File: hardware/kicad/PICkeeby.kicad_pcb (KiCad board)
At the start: 4 copper layers, 85.7 x 55.9 mm, 35 parts, among them J1 PS/2 Connector, J2 PS/2 Connector, J3 MODE_SELECT, J4 Host Interface, J5 Conn_PIC_ICSP_ICD, J6 PS/2 Header, J7 PS/2 Header, U1 PIC16F18344-P, U2 74HCT574, U3 74HCT373, U4 ATF22V10C-10PC

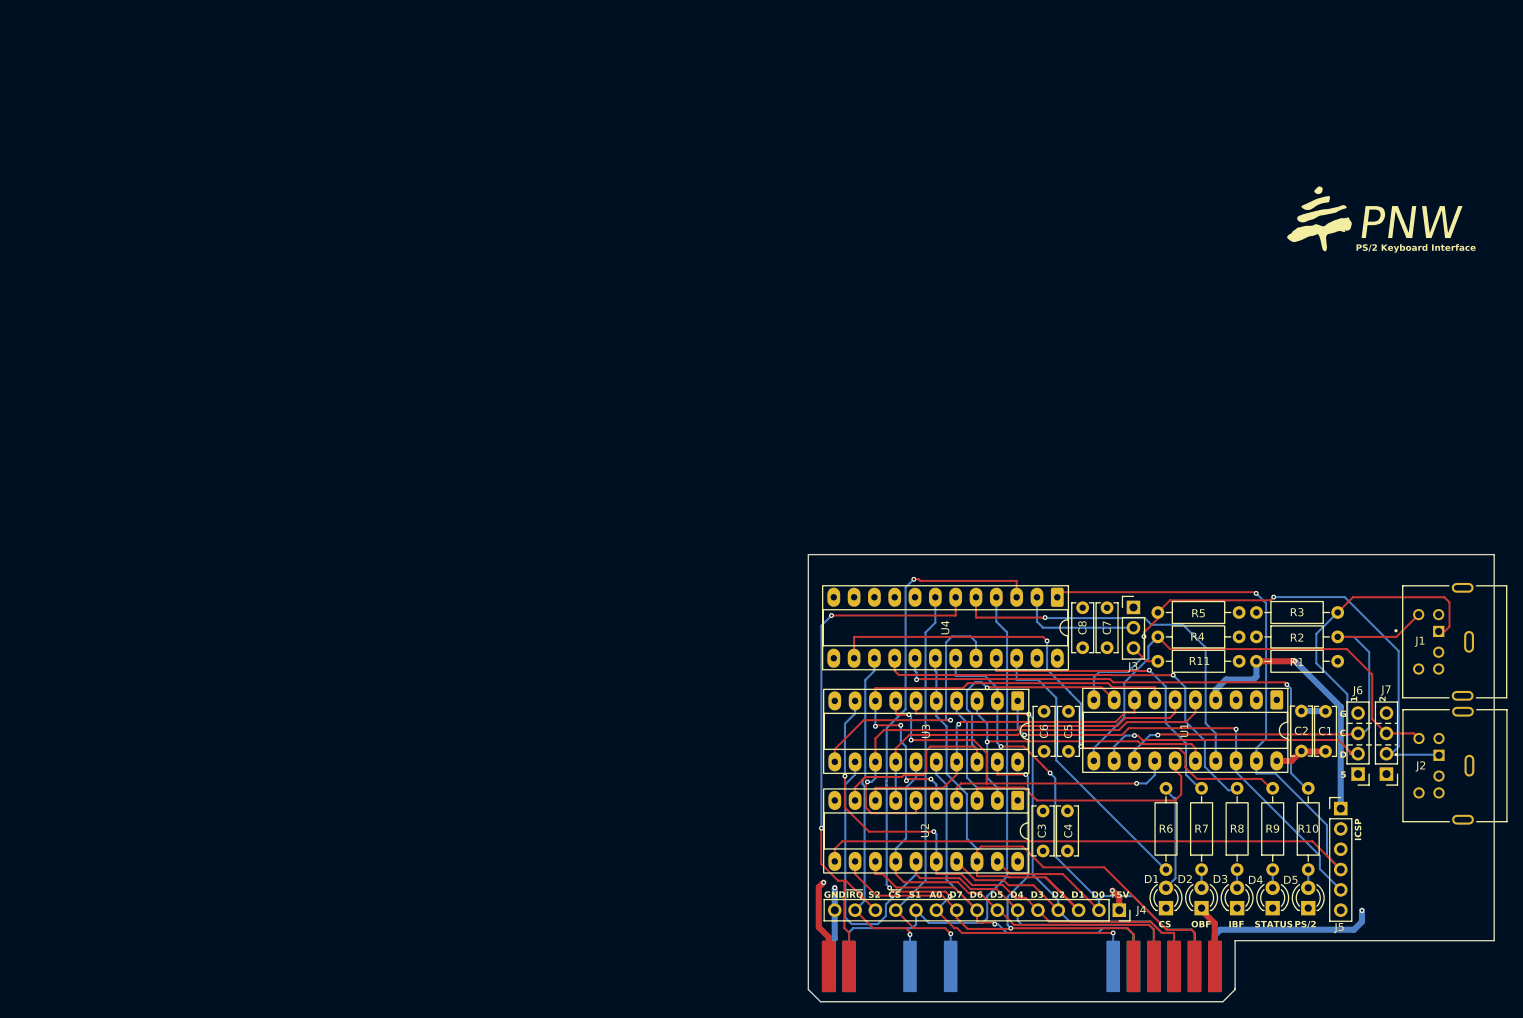
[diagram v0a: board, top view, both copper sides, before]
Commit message: v2
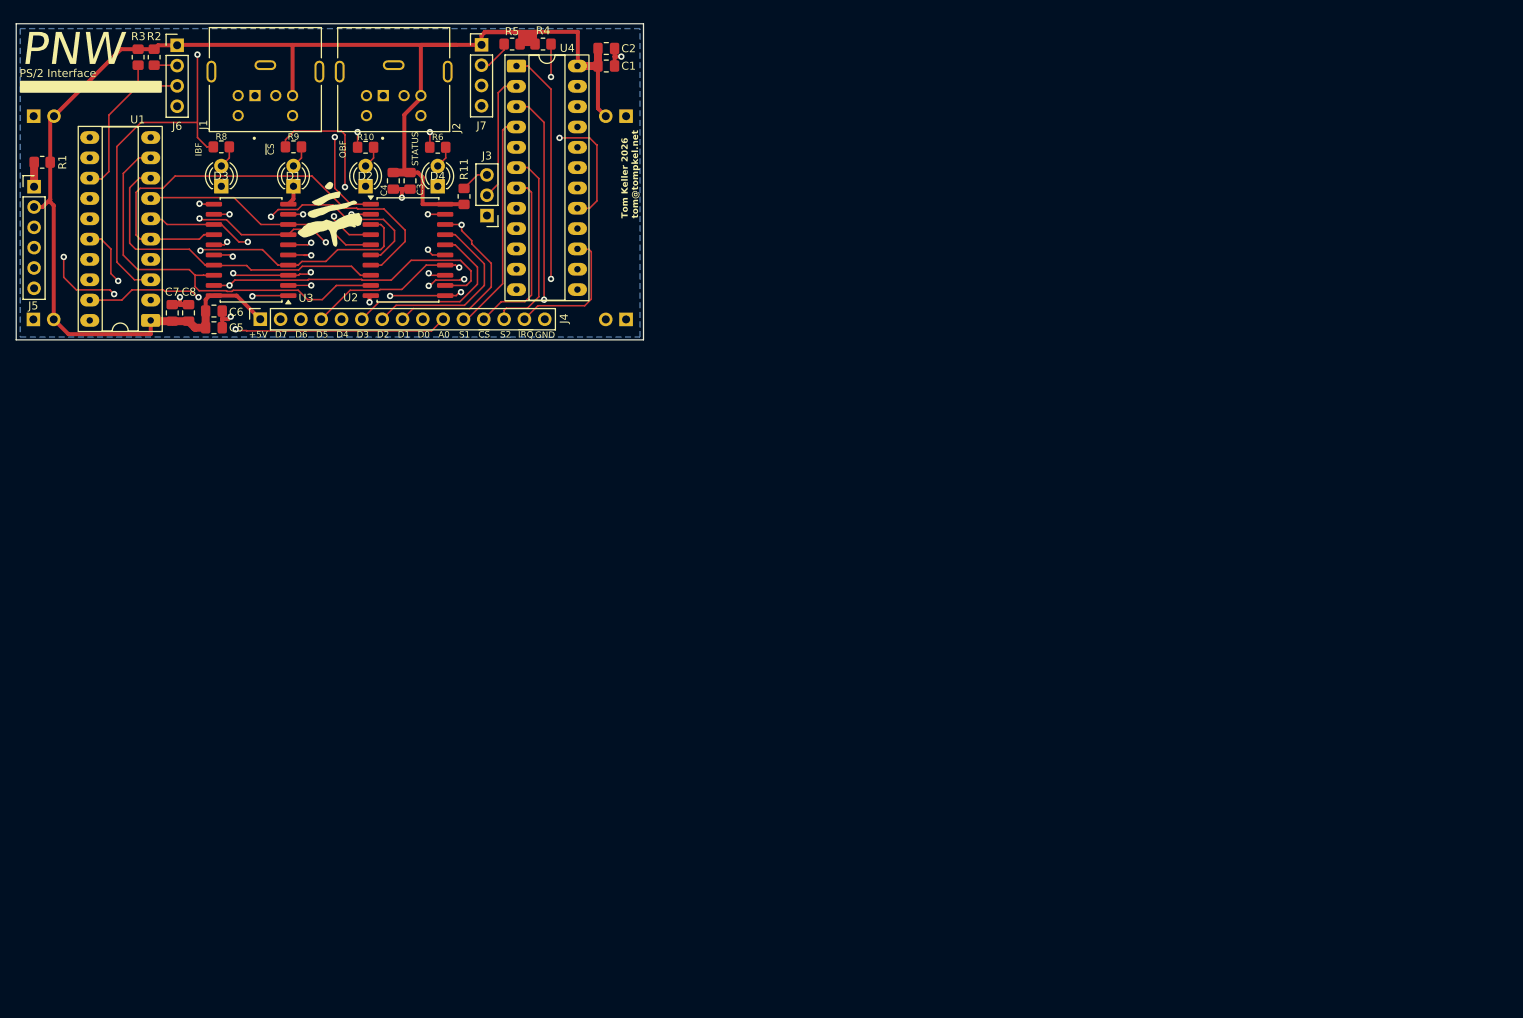
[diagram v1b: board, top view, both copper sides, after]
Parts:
- removed D5: LED, LED_THT:LED_D3.0mm_FlatTop
- removed R7: 470R, Resistor_THT:R_Axial_DIN0207_L6.3mm_D2.5mm_P10.16mm_Horizontal
- added x1: PinHeader_1x02_P2.54mm_Vertical, Connector_PinHeader_2.54mm:PinHeader_1x02_P2.54mm_Vertical, B.Cu at (10.2, 17.9)
- added x2: PinHeader_1x02_P2.54mm_Vertical, Connector_PinHeader_2.54mm:PinHeader_1x02_P2.54mm_Vertical, B.Cu at (10.1, 43.3)
- added x3: PinHeader_1x02_P2.54mm_Vertical, Connector_PinHeader_2.54mm:PinHeader_1x02_P2.54mm_Vertical, B.Cu at (84.2, 17.9)
- added x4: PinHeader_1x02_P2.54mm_Vertical, Connector_PinHeader_2.54mm:PinHeader_1x02_P2.54mm_Vertical, B.Cu at (84.2, 43.3)
- C1, C2, C3, C4, C5, C6, C7, C8: footprint Capacitor_THT:C_Disc_D6.0mm_W2.5mm_P5.00mm -> Capacitor_SMD:C_0805_2012Metric_Pad1.18x1.45mm_HandSolder
- R1, R10, R11, R2, R3, R4, R5, R6, R8, R9: footprint Resistor_THT:R_Axial_DIN0207_L6.3mm_D2.5mm_P10.16mm_Horizontal -> Resistor_SMD:R_0805_2012Metric_Pad1.20x1.40mm_HandSolder
- U2, U3: footprint Package_DIP:DIP-20_W7.62mm_Socket_LongPads -> Package_SO:SOIC-20W_7.5x12.8mm_P1.27mm
- moved J5 180.9 mm to (10.2, 26.7)
- moved R1 173.5 mm to (11.2, 23.7)
- moved J6 173.5 mm to (28.1, 9.04), turned to 0 degrees
- moved J1 166.8 mm to (39.1, 11.5), turned to 180 degrees
- moved R3 163.4 mm to (25.2, 10.5), turned to 90 degrees
- moved J2 160.5 mm to (55.2, 11.5), turned to 180 degrees
- moved R2 157.5 mm to (23.2, 10.5), turned to -90 degrees
- moved R8 155.8 mm to (33.6, 21.7), turned to 180 degrees
- moved D3 155.8 mm to (33.6, 26.7)
- moved R9 152.1 mm to (42.6, 21.7), turned to 180 degrees
- moved U1 148.5 mm to (24.8, 43.4), turned to 180 degrees
- moved R10 148.4 mm to (51.7, 21.8), turned to 180 degrees
- moved J7 145.3 mm to (66.1, 8.99), turned to 0 degrees
- moved D1 141.6 mm to (42.6, 26.7)
- moved D2 138.1 mm to (51.7, 26.7)
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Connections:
- J1 pad S1: GND -> (no net)
- J1 pad S2: GND -> (no net)
- J1 pad S3: GND -> (no net)
- J2 pad S1: GND -> (no net)
- J2 pad S2: GND -> (no net)
- J2 pad S3: GND -> (no net)
- J4 pad 2: /HDATA0 -> /HDATA7
- J4 pad 3: /HDATA1 -> /HDATA6
- J4 pad 4: /HDATA2 -> /HDATA5
- J4 pad 5: /HDATA3 -> /HDATA4
- J4 pad 6: /HDATA4 -> /HDATA3
- J4 pad 7: /HDATA5 -> /HDATA2
- J4 pad 8: /HDATA6 -> /HDATA1
- J4 pad 9: /HDATA7 -> /HDATA0
- J5 pad 1: VPP -> A0
- R1 pad 2: VPP -> A0
- R10 pad 1: Net-(D5-A) -> Net-(D2-A)
- R6 pad 1: Net-(D1-A) -> Net-(D4-A)
- R8 pad 2: Net-(R8-Pad2) -> LED_RX
- R9 pad 1: Net-(D4-A) -> Net-(D1-A)
- U1 pad 4: VPP -> A0
- U2 pad 1: unconnected-(U2-OE-Pad1) -> ~{RD_DATA}
- U4 pad 16: Net-(R8-Pad2) -> LED_RX
- U4 pad 21: Net-(R7-Pad2) -> /HDATA5
- U4 pad 8: GND -> ~{AUX}
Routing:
- net +5V: track 42.1 -> 222.5 mm, vias 3 -> 0
- net LED_RX: track 0.00 -> 115.4 mm, vias 0 -> 1
- net ~{AUX}: track 0.00 -> 60.6 mm
- net Net-(R8-Pad2): track 55.0 -> 0.00 mm, vias 1 -> 0
- net ~{RD_DATA}: track 0.00 -> 45.5 mm, vias 0 -> 1
- net SIG2: track 69.6 -> 24.3 mm, vias 2 -> 0
- net PS2_DATA1: track 77.5 -> 37.0 mm, vias 1 -> 0
- net SIG1: track 66.3 -> 27.4 mm
- net Net-(R7-Pad2): track 38.5 -> 0.00 mm, vias 1 -> 0
- net VPP: track 34.5 -> 0.00 mm, vias 1 -> 0
- net ~{CS}: track 53.4 -> 22.2 mm, vias 1 -> 0
- net /HDATA2: track 76.8 -> 46.4 mm
- net /IDATA3: track 58.5 -> 29.8 mm, vias 4 -> 0
- net ~{IRQ}: track 45.0 -> 17.1 mm, vias 1 -> 0
- net A0: track 93.1 -> 119.5 mm
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- added copper zone on B.Cu, net GND
- removed copper zone on In2.Cu, net +5V
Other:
- board size 85.7 x 55.9 mm -> 78.4 x 39.5 mm
- board text added: "PS/2 Interface"
- board text added: "Tom Keller 2026 tom@tompkel.net"
- board text removed: "1"
- board text removed: "2"
- board text removed: "5"
- board text removed: "C"
- board text removed: "CS"
- board text removed: "D"
- board text removed: "G"
- board text removed: "ICSP"
- board text removed: "PS/2"
- board text removed: "PS/2 Keyboard Interface"
